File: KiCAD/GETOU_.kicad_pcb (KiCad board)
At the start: 2 copper layers, 106.5 x 58 mm, 25 parts, among them U1 XIAO-RP2040-DIP

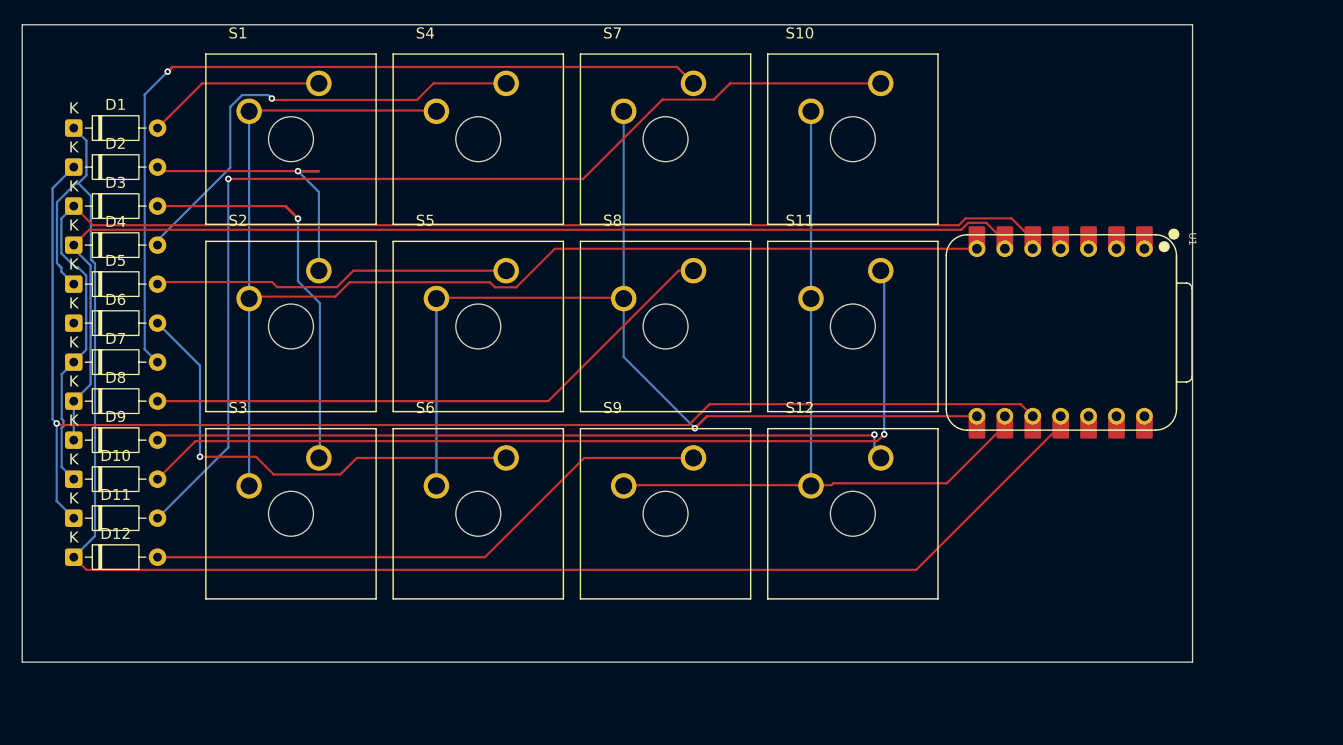
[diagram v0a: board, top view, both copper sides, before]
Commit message: Add and modify files
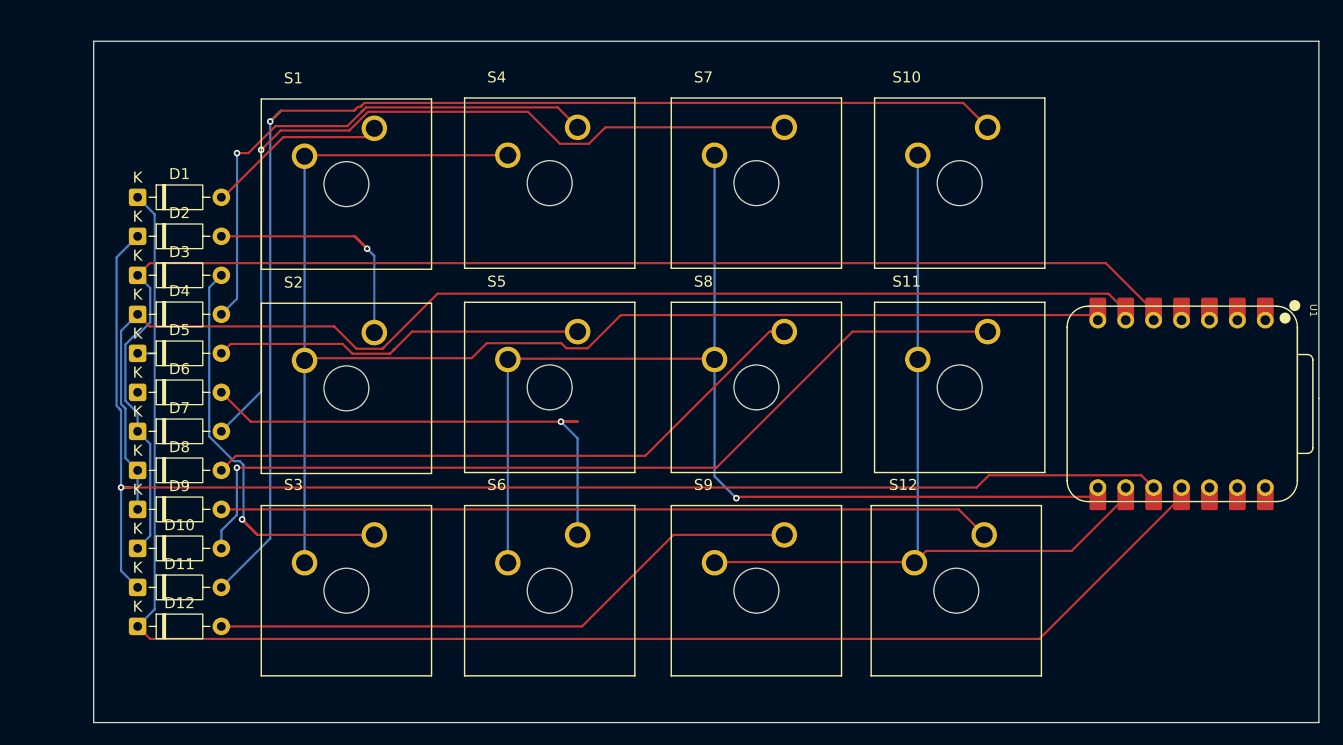
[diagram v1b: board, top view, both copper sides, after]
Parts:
- moved U1 12.8 mm to (191.0, 93.5)
- moved S12 11.7 mm to (170.5, 110.5)
- moved S11 11.2 mm to (170.8, 92.0)
- moved S9 10.8 mm to (152.3, 110.5)
- moved S10 10.5 mm to (170.8, 73.4)
- moved S8 9.95 mm to (152.3, 92.0)
- moved S6 9.55 mm to (133.5, 110.5)
- moved S7 9.18 mm to (152.3, 73.4)
- moved S3 8.63 mm to (115.0, 110.5)
- moved D10 8.57 mm to (96.0, 106.7)
- moved D5 8.57 mm to (96.0, 88.9)
- moved D1 8.57 mm to (96.0, 74.7)
- moved D11 8.57 mm to (96.0, 110.2)
- moved D12 8.57 mm to (96.0, 113.8)
- moved D2 8.57 mm to (96.0, 78.2)
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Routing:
- net Net-(D11-A): track 96.5 -> 114.3 mm
- net row0: track 120.5 -> 130.7 mm
- net col3: track 106.2 -> 114.2 mm
- net col1: track 124.5 -> 131.3 mm
- net Net-(D4-A): track 42.4 -> 49.0 mm
- net Net-(D6-A): track 42.9 -> 49.0 mm
- net col2: track 117.8 -> 123.4 mm
- net col0: track 149.0 -> 143.5 mm
- net row2: track 73.6 -> 78.0 mm
- net row1: track 98.8 -> 103.2 mm
- net Net-(D8-A): track 53.7 -> 56.5 mm
- net Net-(D9-A): track 67.8 -> 70.4 mm, vias 1 -> 0
- net Net-(D3-A): track 42.4 -> 44.9 mm
- net Net-(D2-A): track 30.4 -> 28.0 mm
- net Net-(D12-A): track 52.5 -> 54.7 mm
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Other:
- board size 106.5 x 58 mm -> 111.5 x 62 mm
